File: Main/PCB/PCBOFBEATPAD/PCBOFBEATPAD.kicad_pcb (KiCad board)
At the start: 2 copper layers, 112.7 x 121.4 mm, 51 parts, among them J2 7_pin_conector, SW1 SW_Push, U4 ESP32-C3_SUPERMINI_TH

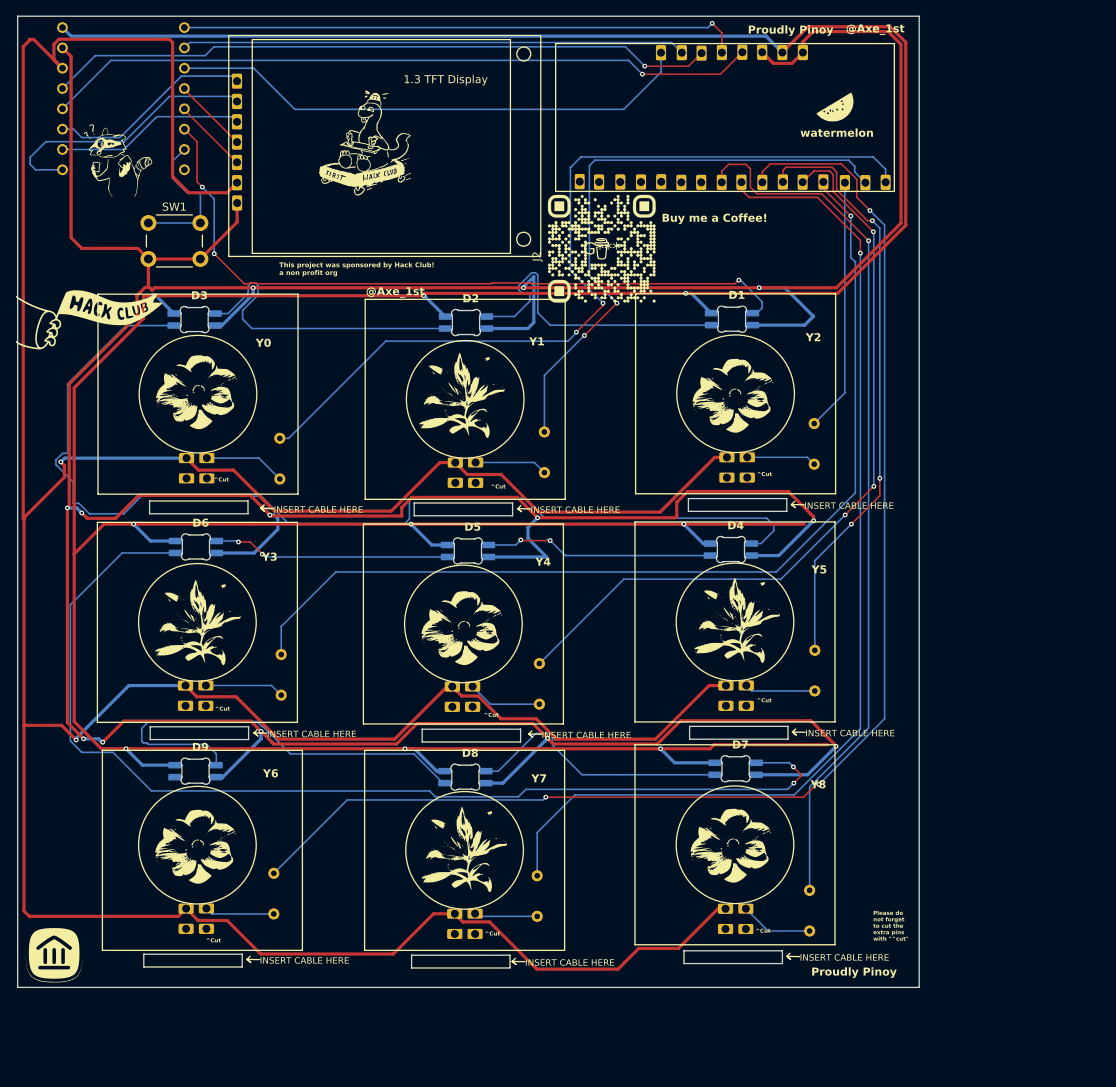
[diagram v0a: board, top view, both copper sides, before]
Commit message: Major Update (V2 RELEASE)
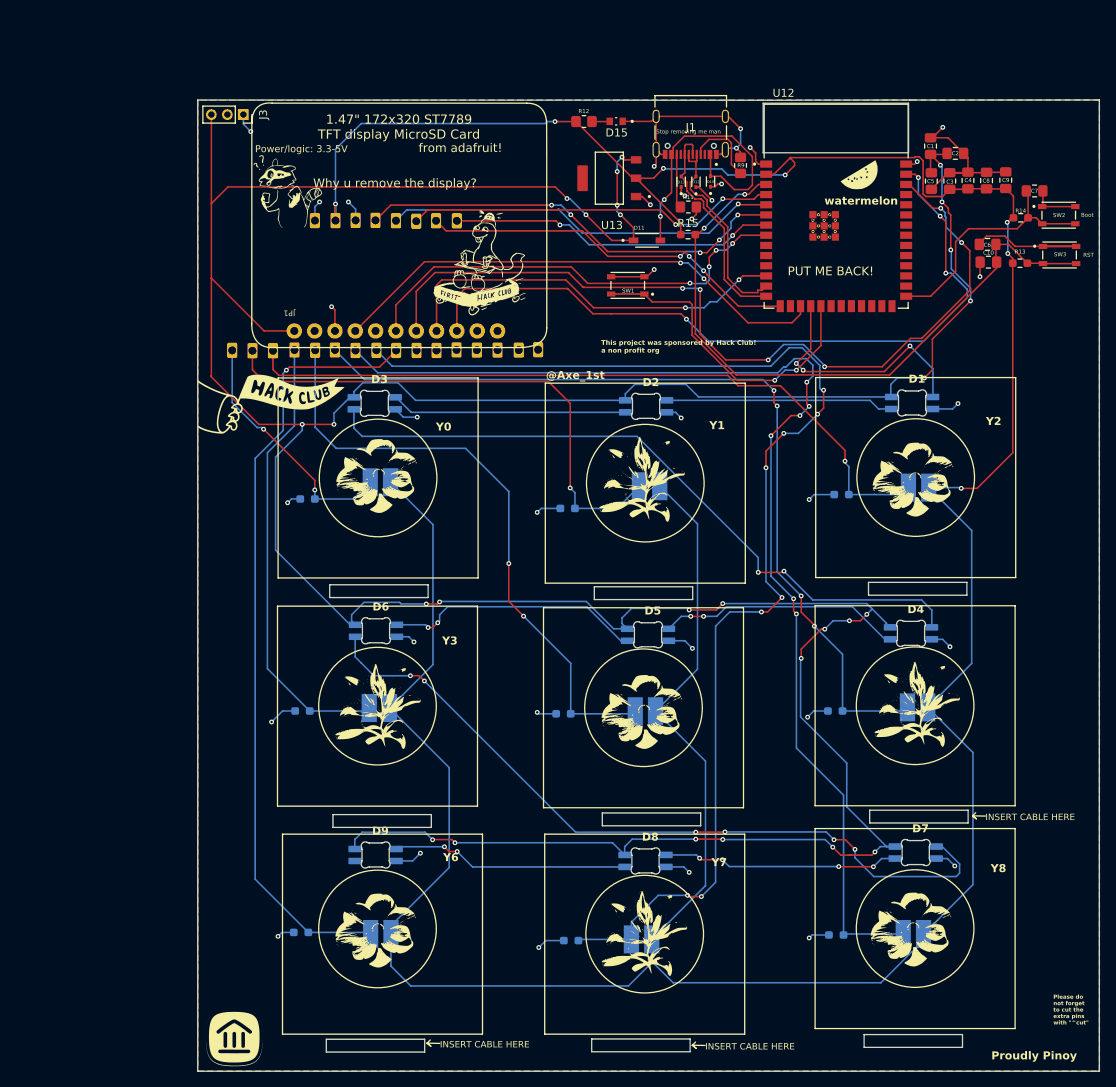
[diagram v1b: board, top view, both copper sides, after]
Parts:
- removed A1, A2, A3, A4, A5, A6, A7, A8, A9: ~, ESP32-C3_SUPERMINI_TH:2x2 connectorss
- removed the G*** at (79.7, 135.8)
- removed the G*** at (66.2, 69.7)
- removed the G*** at (69.8, 49.7)
- removed the G*** at (130.3, 60.9)
- removed the G*** at (79.8, 79.0)
- removed the G*** at (146.6, 135.7)
- removed the G*** at (111.8, 135.9)
- removed the G*** at (77.6, 133.8)
- removed the G*** at (160.7, 60.5)
- removed the G*** at (156.2, 143.6)
- removed the G*** at (129.8, 42.0)
- removed the G*** at (111.5, 79.1)
- removed the G*** at (158.7, 42.9)
- removed the G*** at (61.8, 148.9)
- removed the G*** at (78.5, 107.5)
- removed the G*** at (159.4, 43.1)
- removed the G*** at (113.0, 108.5)
- removed the G*** at (145.9, 107.2)
- removed the G*** at (146.8, 79.5)
- removed the G*** at (100.7, 47.6)
- removed J2: 7_pin_conector, ESP32-C3_SUPERMINI_TH:1.3 tft display
- removed U4: ESP32-C3_SUPERMINI_TH, ESP32-C3_SUPERMINI_TH:MODULE_ESP32-C3_SUPERMINI_TH
- added C1: 10uF, Capacitor_SMD:C_0805_2012Metric_Pad1.18x1.45mm_HandSolder, F.Cu at (171.4, 48.0)
- added C10: 1uF, Capacitor_SMD:C_0805_2012Metric_Pad1.18x1.45mm_HandSolder, F.Cu at (178.6, 62.5)
- added C2: 10uF, Capacitor_SMD:C_0805_2012Metric_Pad1.18x1.45mm_HandSolder, F.Cu at (174.5, 48.9)
- added C3: 0u1F, Capacitor_SMD:C_0805_2012Metric_Pad1.18x1.45mm_HandSolder, F.Cu at (173.8, 52.4)
- added C4: 10uF, Capacitor_SMD:C_0805_2012Metric_Pad1.18x1.45mm_HandSolder, F.Cu at (176.0, 52.3)
- added C5: 0u1F, Capacitor_SMD:C_0805_2012Metric_Pad1.18x1.45mm_HandSolder, F.Cu at (171.5, 52.4)
- added C6: 0u1F, Capacitor_SMD:C_0805_2012Metric_Pad1.18x1.45mm_HandSolder, F.Cu at (178.5, 60.3)
- added C7: 0u1F, Capacitor_SMD:C_0805_2012Metric_Pad1.18x1.45mm_HandSolder, F.Cu at (184.4, 53.6)
- added C8: 0u1F, Capacitor_SMD:C_0805_2012Metric_Pad1.18x1.45mm_HandSolder, F.Cu at (178.4, 52.3)
- added C9: 10uF, Capacitor_SMD:C_0805_2012Metric_Pad1.18x1.45mm_HandSolder, F.Cu at (180.8, 52.3)
- added D10: LESD5D5.0CT1G, LESD5D5.0CT1G:TVS_LESD5D5.0CT1G, F.Cu at (143.9, 52.4)
- added D11: 1N5819HW-7-F, 1N5819HW-7-F:SOD3715X145N, F.Cu at (135.9, 59.8)
- added D12: LESD5D5.0CT1G, LESD5D5.0CT1G:TVS_LESD5D5.0CT1G, F.Cu at (142.0, 52.5)
- added D13: LESD5D5.0CT1G, LESD5D5.0CT1G:TVS_LESD5D5.0CT1G, F.Cu at (140.2, 52.5)
- added D15: LTST-C190KGKT, LTST-C190KGKT:LEDC1608X35N, F.Cu at (132.1, 44.9)
- added G***: LOGO, LOGO, F.Cu at (102.2, 146.3)
- added G***: LOGO, LOGO, F.Cu at (91.0, 53.6)
- added G***: LOGO, LOGO, F.Cu at (162.5, 51.6)
- added G***: LOGO, LOGO, F.Cu at (88.9, 80.2)
- added G***: LOGO, LOGO, F.Cu at (102.3, 89.5)
- added G***: LOGO, LOGO, F.Cu at (101.0, 118.0)
- added G***: LOGO, LOGO, B.Cu at (100.1, 144.3)
- added G***: LOGO, LOGO, B.Cu at (158.9, 57.8)
- added G***: LOGO, LOGO, B.Cu at (183.2, 71.0)
- added G***: LOGO, LOGO, F.Cu at (169.1, 146.2)
- added G***: LOGO, LOGO, F.Cu at (134.0, 89.6)
- added G***: LOGO, LOGO, F.Cu at (134.3, 146.3)
- added G***: LOGO, LOGO, F.Cu at (135.5, 119.0)
- added G***: LOGO, LOGO, F.Cu at (168.4, 117.7)
- added G***: LOGO, LOGO, F.Cu at (169.4, 90.0)
- added G***: LOGO, LOGO, F.Cu at (84.3, 159.4)
- added G***: LOGO, LOGO, F.Cu at (115.0, 62.6)
- added J1: TYPE-C-31-M-12, TYPE-C-31-M-12:HRO_TYPE-C-31-M-12, F.Cu at (141.4, 44.3)
- added J3: Conn_01x03, Connector_PinSocket_2.00mm:PinSocket_1x03_P2.00mm_Vertical, F.Cu at (85.5, 44.1)
- added JP1: ~, Adafruit:1X11_ROUND_76, F.Cu at (104.5, 71.1)
- added R10: 10k, Resistor_SMD:R_0603_1608Metric_Pad0.98x0.95mm_HandSolder, B.Cu at (93.5, 92.1)
- added R11: 5k1, Resistor_SMD:R_0805_2012Metric_Pad1.20x1.40mm_HandSolder, F.Cu at (141.1, 55.6)
- added R12: 75, Resistor_SMD:R_0805_2012Metric_Pad1.20x1.40mm_HandSolder, F.Cu at (128.1, 45.0)
- added R13: 10k, Resistor_SMD:R_0603_1608Metric_Pad0.98x0.95mm_HandSolder, F.Cu at (182.6, 62.7)
- added R14: 10k, Resistor_SMD:R_0603_1608Metric_Pad0.98x0.95mm_HandSolder, F.Cu at (182.6, 57.0)
- added R15: 10k, Resistor_SMD:R_0603_1608Metric_Pad0.98x0.95mm_HandSolder, F.Cu at (141.1, 59.1)
- added SW2: PTS810_SJM_250_SMTR_LFS, BUTTONS:SW_PTS810_SJM_250_SMTR_LFS, F.Cu at (187.4, 56.7)
- added SW3: PTS810_SJM_250_SMTR_LFS, BUTTONS:SW_PTS810_SJM_250_SMTR_LFS, F.Cu at (187.5, 61.6)
- added U1: ~, randomahhconnector:2 pin connector, B.Cu at (102.6, 82.8)
- added U10: ~, randomahhconnector:2 pin connector, B.Cu at (135.3, 140.0)
- added U11: ~, randomahhconnector:2 pin connector, B.Cu at (102.7, 139.3)
- added U12: ESP32-S3-WROOM-1-N16R2, ESP32-S3-WROOM-1-N16R2:XCVR_ESP32-S3-WROOM-1-N16R2, F.Cu at (159.6, 55.5)
- added U13: AMS1117-3.3, AMS1117-3.3:SOT229P700X180-4N, F.Cu at (131.2, 52.0)
- added U3: ~, randomahhconnector:2 pin connector, B.Cu at (136.3, 83.3)
- added U5: ~, randomahhconnector:2 pin connector, B.Cu at (169.9, 83.5)
- added U6: ~, randomahhconnector:2 pin connector, B.Cu at (102.5, 111.0)
- added U7: ~, randomahhconnector:2 pin connector, B.Cu at (135.7, 111.4)
- added U8: ~, randomahhconnector:2 pin connector, B.Cu at (169.8, 111.0)
- added U9: ~, randomahhconnector:2 pin connector, B.Cu at (169.2, 139.3)
- R1, R2, R3, R4, R5, R6, R7, R8: value R_Small -> 10k; footprint Resistor_THT:R_Axial_DIN0204_L3.6mm_D1.6mm_P5.08mm_Horizontal -> Resistor_SMD:R_0603_1608Metric_Pad0.98x0.95mm_HandSolder
- R9: value R_Small -> 5k1; footprint Resistor_THT:R_Axial_DIN0204_L3.6mm_D1.6mm_P5.08mm_Horizontal -> Resistor_SMD:R_0805_2012Metric_Pad1.20x1.40mm_HandSolder; moved to F.Cu
- SW1: value SW_Push -> PTS810_SJM_250_SMTR_LFS; footprint Button_Switch_THT:SW_PUSH_6mm -> BUTTONS:SW_PTS810_SJM_250_SMTR_LFS
- U2: moved to B.Cu
- moved R9 91.0 mm to (147.6, 50.4), turned to 90 degrees
- moved U2 86.5 mm to (83.0, 74.7)
- moved R8 73.3 mm to (92.7, 146.3), turned to 180 degrees
- moved R2 72.8 mm to (160.2, 91.6), turned to 180 degrees
- moved R7 71.4 mm to (126.4, 147.3), turned to 180 degrees
- moved SW1 60.4 mm to (133.5, 65.4), turned to 180 degrees
- moved R6 38.1 mm to (159.6, 146.6), turned to 180 degrees
- moved R5 37.5 mm to (159.5, 118.6), turned to 180 degrees
- moved R1 37.0 mm to (126.0, 93.3), turned to 180 degrees
- moved R4 35.3 mm to (125.5, 119.0), turned to 180 degrees
- moved D4 24.8 mm to (168.9, 109.0)
- moved D3 24.8 mm to (101.9, 80.3)
- moved D5 24.8 mm to (136.0, 109.2)
- moved D9 24.8 mm to (102.0, 136.7)
- moved D8 24.8 mm to (135.7, 137.5)
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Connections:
- D1 pad 1: VCC -> VCC_5V
- D2 pad 1: VCC -> VCC_5V
- D3 pad 1: VCC -> VCC_5V
- D4 pad 1: VCC -> VCC_5V
- D5 pad 1: VCC -> VCC_5V
- D6 pad 1: VCC -> VCC_5V
- D7 pad 1: VCC -> VCC_5V
- D8 pad 1: VCC -> VCC_5V
- D9 pad 1: VCC -> VCC_5V
- R1 pad 1: Y0 -> Y1
- R1 pad 2: Net-(A1-Pin_1) -> GND
- R2 pad 1: Y3 -> Y2
- R2 pad 2: Net-(A4-Pin_1) -> GND
- R3 pad 1: Y6 -> Y3
- R3 pad 2: Net-(A7-Pin_1) -> GND
- R4 pad 1: Y1 -> Y4
- R4 pad 2: Net-(A2-Pin_1) -> GND
- R5 pad 1: Y4 -> Y5
- R5 pad 2: Net-(A5-Pin_1) -> GND
- R6 pad 1: Y7 -> Y6
- R6 pad 2: Net-(A8-Pin_1) -> GND
- R7 pad 1: Y2 -> Y7
- R7 pad 2: Net-(A3-Pin_1) -> GND
- R8 pad 1: Y5 -> Y8
- R8 pad 2: Net-(A6-Pin_1) -> GND
- R9 pad 1: Y8 -> Net-(J1-CC1)
- R9 pad 2: Net-(A9-Pin_1) -> GND
- SW1 pad 1: Net-(U4-GPIO20) -> SW_PUSH
- SW1 pad 2: GND -> SW_PUSH
- U2 pad 2: VCC -> 3.3v
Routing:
- net VCC: track 525.1 -> 0.00 mm, vias 9 -> 0
- net VCC_5V: track 0.00 -> 473.3 mm, vias 0 -> 27
- net GND: track 562.7 -> 137.0 mm, vias 13 -> 35
- net CS_DISPLAY: track 0.00 -> 106.2 mm, vias 0 -> 6
- net DC_DISPLAY: track 0.00 -> 93.1 mm, vias 0 -> 4
- net CHIP_PU: track 0.00 -> 83.2 mm, vias 0 -> 2
- net Y0: track 108.6 -> 31.0 mm
- net Y3: track 122.7 -> 56.3 mm, vias 1 -> 0
- net SCK_DISPLAY: track 0.00 -> 63.9 mm, vias 0 -> 2
- net Y2: track 31.7 -> 91.6 mm, vias 0 -> 1
- net SK MINI LED: track 90.8 -> 31.8 mm
- net MOSI_DISPLAY: track 0.00 -> 56.6 mm, vias 0 -> 4
- net RST: track 0.00 -> 50.3 mm, vias 0 -> 2
- net Net-(D3-DOUT): track 132.0 -> 87.4 mm, vias 0 -> 2
- net SW_PUSH: track 0.00 -> 39.7 mm, vias 0 -> 2
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- added copper zone on B.Cu, net GND
- added copper zone on F.Cu, net GND
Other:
- outline, holes or cut-outs redrawn
- board text added: "1.47" 172x320 ST7789 TFT display MicroSD Card"
- board text added: "Boot"
- board text added: "PUT ME BACK!"
- board text added: "Power/logic: 3.3-5V"
- board text added: "RST"
- board text added: "Stop removing me man"
- board text added: "Why u remove the display?"
- board text added: "from adafruit!"
- board text removed: "Plug Flex here>"
- board text removed: "These are live!"
- board text removed: "XIAO HERE"
- board text removed: "Y4"
- board text removed: "Y5"
- board text removed: "^Cut"
